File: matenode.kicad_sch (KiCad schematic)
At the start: 79 parts, among them J1 USB_C_Receptacle, J10 BAT_CONN, J2 VIN, J3 QWIIC, J4 VIN, J5 Lichtenprog_conn, J6 VIN, J7 VIN, J8 VIN, J9 SPK_OUT, Q1 MMBT2222A, Q2 MMBT2222A, Q3 BSS84, Q4 MMBT2222A, SW2 RST, SW3 B2, SW4 BOOT/B1, U1 SPX3819M5-L-3-3, U2 BQ24073RGT, U3 JLC_OLED, U4 ESP32-C3-WROOM-02, U5 PAM8302AAD

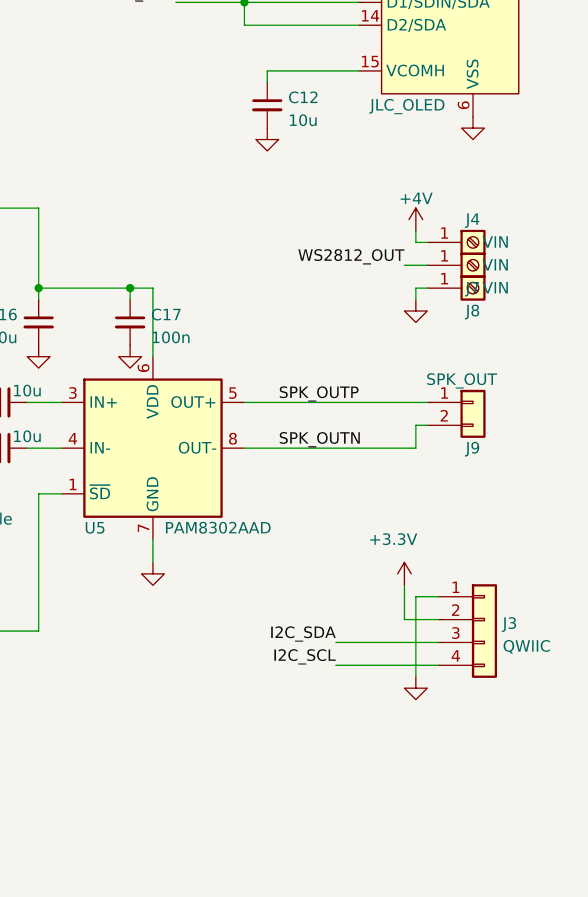
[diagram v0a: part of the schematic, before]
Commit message: final final
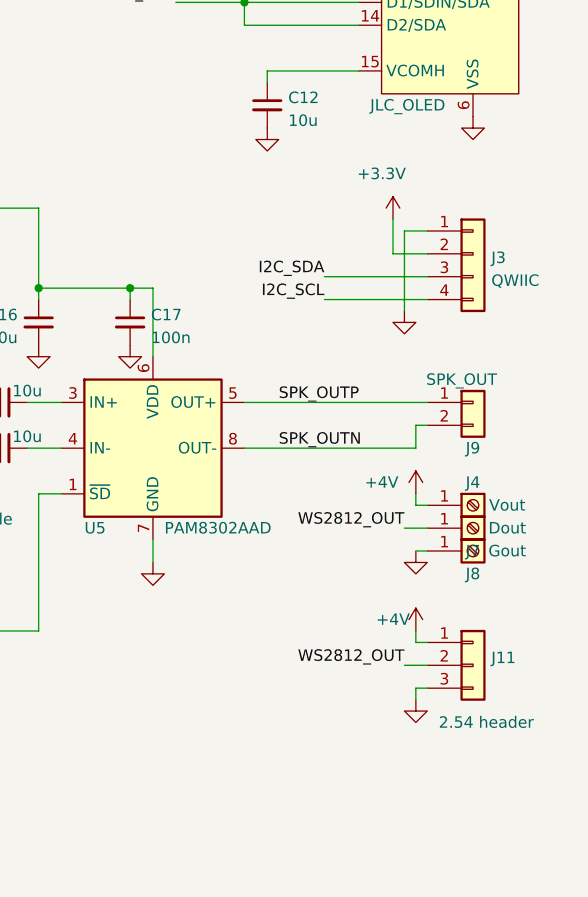
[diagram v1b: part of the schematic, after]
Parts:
- added J11: 2.54 header, Connector_PinHeader_2.54mm:PinHeader_1x03_P2.54mm_Vertical, symbol Connector_Generic:Conn_01x03
- J4: value VIN -> Vout
- J7: value VIN -> Dout
- J8: value VIN -> Gout
- R12, R13, R14: footprint Resistor_SMD:R_0402_1005Metric -> Resistor_SMD:R_0603_1608Metric
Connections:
- net +4V: now also J11.1 (Pin_1)
- net GND: now also J11.3 (Pin_3)
- net WS2812_OUT: now also J11.2 (Pin_2)
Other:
- moved on the sheet: J3, J4, J7, J8
